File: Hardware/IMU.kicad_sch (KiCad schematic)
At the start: 2 parts, among them J2 Conn_01x04_Socket, J4 Conn_01x08_Socket

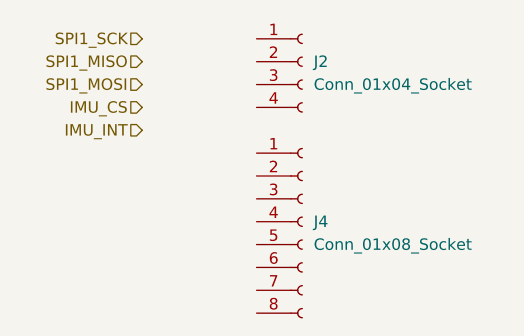
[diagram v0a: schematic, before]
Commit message: Updated: ERC fixes
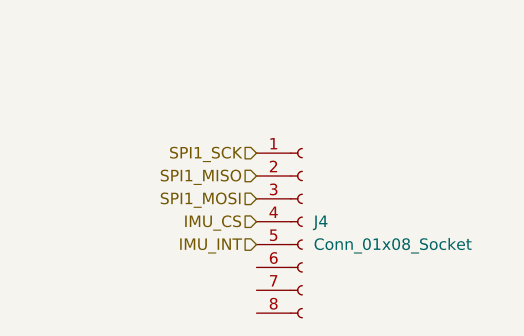
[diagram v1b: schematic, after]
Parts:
- removed J2: Conn_01x04_Socket, symbol Connector:Conn_01x04_Socket
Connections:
- net IMU_CS: now also J4.4 (Pin_4)
- net IMU_INT: now also J4.5 (Pin_5)
- net SPI1_MISO: now also J4.2 (Pin_2)
- net SPI1_MOSI: now also J4.3 (Pin_3)
- net SPI1_SCK: now also J4.1 (Pin_1)
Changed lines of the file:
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@@
 	(hierarchical_label "SPI1_MOSI"
 		(shape input)
-		(at 106.68 87.63 180)
+		(at 119.38 100.33 180)
 		(effects
 			(font
@@
 	(hierarchical_label "IMU_INT"
 		(shape input)
-		(at 106.68 92.71 180)
+		(at 119.38 105.41 180)
 		(effects
 			(font
@@
 	(hierarchical_label "SPI1_MISO"
 		(shape input)
-		(at 106.68 85.09 180)
+		(at 119.38 97.79 180)
 		(effects
 			(font
@@
 	(hierarchical_label "SPI1_SCK"
 		(shape input)
-		(at 106.68 82.55 180)
+		(at 119.38 95.25 180)
 		(effects
 			(font
@@
 	(hierarchical_label "IMU_CS"
 		(shape input)
-		(at 106.68 90.17 180)
+		(at 119.38 102.87 180)
 		(effects
 			(font
@@
 		)
 	)
-	(symbol
-		(lib_id "Connector:Conn_01x04_Socket")
-		(at 124.46 85.09 0)
-		(unit 1)
-		(exclude_from_sim no)
-		(in_bom yes)
-		(on_board yes)
-		(dnp no)
-		(fields_autoplaced yes)
-		(property "Reference" "J2"
-			(at 125.73 85.0899 0)
-			(effects
-				(font
-					(size 1.27 1.27)
-				)
-				(justify left)
-			)
-		)
-		(property "Value" "Conn_01x04_Socket"
-			(at 125.73 87.6299 0)
-			(effects
-				(font
-					(size 1.27 1.27)
-				)
-				(justify left)
-			)
-		)
-		(property "Footprint" ""
-			(at 124.46 85.09 0)
-			(effects
-				(font
-					(size 1.27 1.27)
-				)
-				(hide yes)
-			)
-		)
-		(property "Datasheet" "~"
-			(at 124.46 85.09 0)
-			(effects
-				(font
-					(size 1.27 1.27)
-				)
-				(hide yes)
-			)
-		)
-		(property "Description" "Generic connector, single row, 01x04, script generated"
-			(at 124.46 85.09 0)
-			(effects
-				(font
-					(size 1.27 1.27)
-				)
-				(hide yes)
-			)
-		)
-		(pin "4"
-		)
-		(pin "3"
-		)
-		(pin "2"
-		)
-		(pin "1"
-		)
-		(instances
-			(project ""
-				(path "/16e232dd-2018-4914-997b-dd1e00d4fd91/dbc3c749-3435-48d4-acdf-7af82590aef3"
-					(reference "J2")
-					(unit 1)
-				)
-			)
-		)
-	)
